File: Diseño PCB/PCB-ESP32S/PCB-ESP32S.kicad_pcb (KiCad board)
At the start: 2 copper layers, 29 parts, among them J1 Conn_01x04, J7 Screw_Terminal_01x03, J8 Screw_Terminal_01x02, Q3 TIP42C, SW1 SW_DIP_x01, SW2 SW_DIP_x01, U1 ESP-32S, U5 LM7805_TO220, U6 LM1117-3.3, u2 Conn_01x04_Male, u7 Conn_01x04_Male

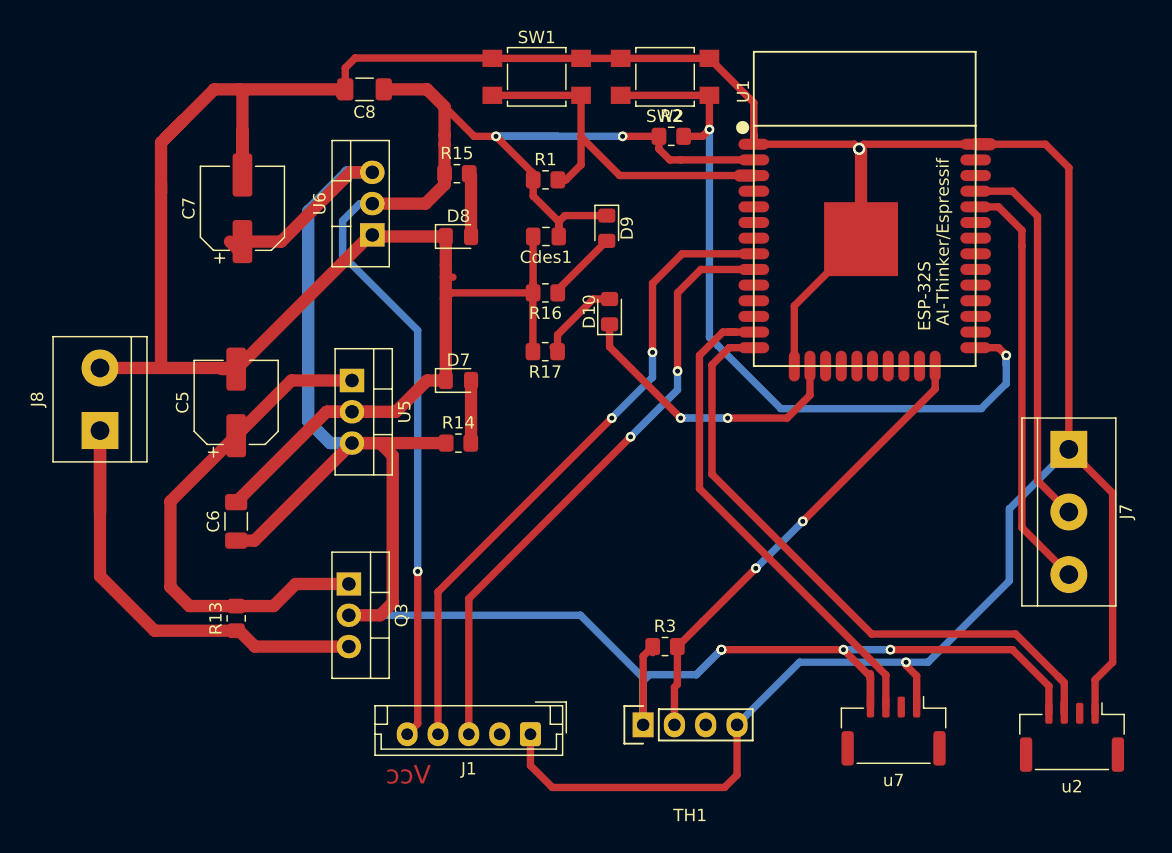
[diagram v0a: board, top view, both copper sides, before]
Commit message: pcv v2
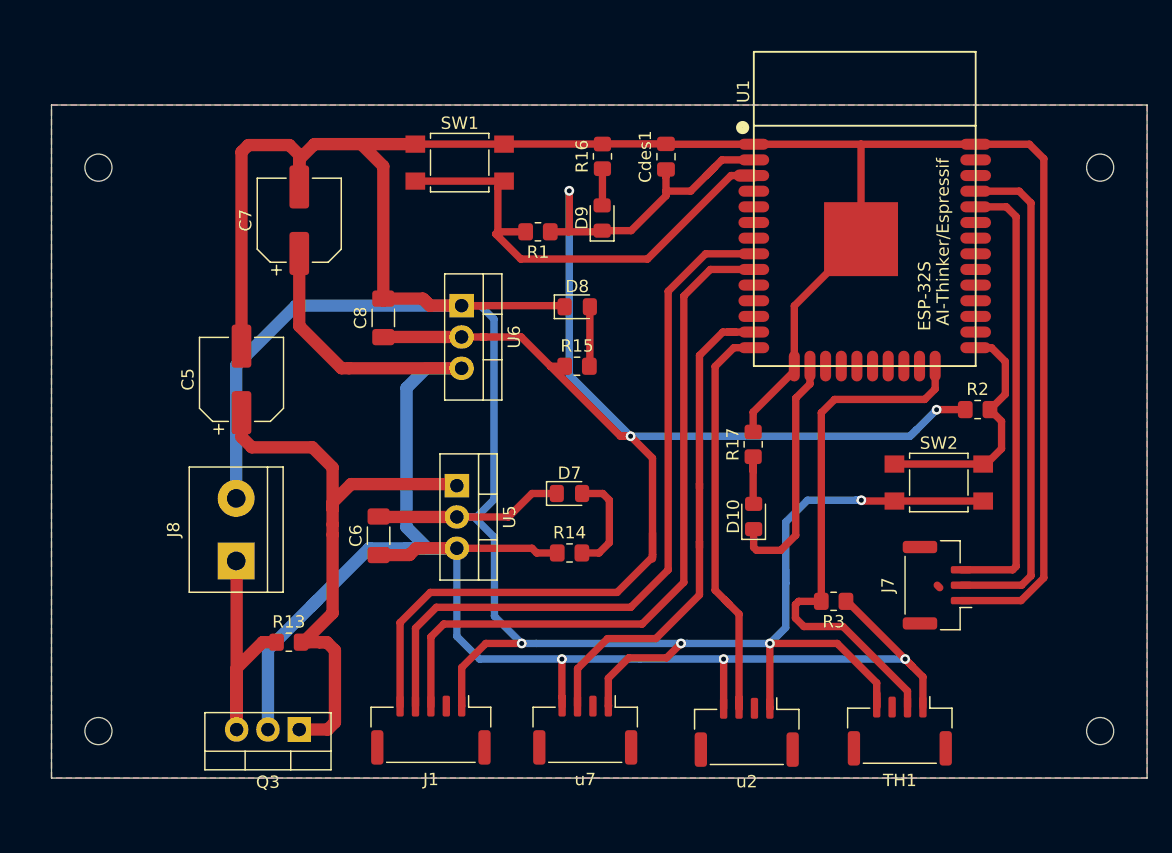
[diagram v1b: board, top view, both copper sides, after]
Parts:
- added ?: MountingHole_2.2mm_M2, MountingHole:MountingHole_2.2mm_M2, F.Cu at (243.8, 80.0)
- added ?: MountingHole_2.2mm_M2, MountingHole:MountingHole_2.2mm_M2, F.Cu at (243.8, 125.7)
- added ?: MountingHole_2.2mm_M2, MountingHole:MountingHole_2.2mm_M2, F.Cu at (162.6, 125.7)
- added ?: MountingHole_2.2mm_M2, MountingHole:MountingHole_2.2mm_M2, F.Cu at (162.6, 80.0)
- J1: footprint Connector_JST:JST_EH_B5B-EH-A_1x05_P2.50mm_Vertical -> Connector_JST:JST_GH_BM05B-GHS-TBT_1x05-1MP_P1.25mm_Vertical
- J7: footprint TerminalBlock:TerminalBlock_bornier-3_P5.08mm -> Connector_JST:JST_GH_BM03B-GHS-TBT_1x03-1MP_P1.25mm_Vertical
- TH1: footprint Sensors:DHT22_Temperature_Humidity -> Connector_JST:JST_GH_BM04B-GHS-TBT_1x04-1MP_P1.25mm_Vertical
- moved SW2 39.7 mm to (230.7, 105.6), turned to 0 degrees
- moved R2 33.3 mm to (233.9, 99.6)
- moved u2 26.4 mm to (215.2, 125.8)
- moved u7 25.0 mm to (202.1, 125.7)
- moved D10 20.3 mm to (215.7, 108.3)
- moved C8 18.6 mm to (185.7, 92.2), turned to 90 degrees
- moved R17 18.5 mm to (215.7, 102.5), turned to 90 degrees
- moved R15 18.4 mm to (201.4, 96.1)
- moved TH1 17.0 mm to (227.6, 125.7), turned to 180 degrees
- moved J7 15.3 mm to (230.6, 113.9), turned to 90 degrees
- moved J8 15.3 mm to (173.7, 111.9)
- moved R3 14.2 mm to (222.2, 115.2), turned to 180 degrees
- moved D7 12.9 mm to (200.8, 106.5)
- moved R14 12.7 mm to (200.8, 111.3)
- moved Q3 12.5 mm to (178.9, 125.6), turned to 180 degrees
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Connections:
- J1 pad 2: /BH1750/ADDR -> (no net)
- TH1 pad 3: Net-(TH1-Pad3) -> (no net)
- U1 pad 10: Net-(U1-Pad10) -> (no net)
- U1 pad 11: Net-(U1-Pad11) -> (no net)
- U1 pad 12: Net-(U1-Pad12) -> (no net)
- U1 pad 17: Net-(U1-Pad17) -> (no net)
- U1 pad 18: Net-(U1-Pad18) -> (no net)
- U1 pad 19: Net-(U1-Pad19) -> (no net)
- U1 pad 20: Net-(U1-Pad20) -> (no net)
- U1 pad 21: Net-(U1-Pad21) -> (no net)
- U1 pad 22: Net-(U1-Pad22) -> (no net)
- U1 pad 23: Net-(U1-Pad23) -> (no net)
- U1 pad 26: Net-(U1-Pad26) -> (no net)
- U1 pad 27: Net-(U1-Pad27) -> (no net)
- U1 pad 28: Net-(U1-Pad28) -> (no net)
- U1 pad 29: Net-(U1-Pad29) -> (no net)
- U1 pad 30: Net-(U1-Pad30) -> (no net)
- U1 pad 31: Net-(U1-Pad31) -> (no net)
- U1 pad 32: Net-(U1-Pad32) -> (no net)
- U1 pad 33: Net-(U1-Pad33) -> (no net)
- U1 pad 36: Net-(U1-Pad36) -> (no net)
- U1 pad 37: Net-(U1-Pad37) -> (no net)
- U1 pad 4: Net-(U1-Pad4) -> (no net)
- U1 pad 5: Net-(U1-Pad5) -> (no net)
- U1 pad 6: Net-(U1-Pad6) -> (no net)
- U1 pad 7: Net-(U1-Pad7) -> (no net)
- u2 pad 2: Net-(u2-Pad2) -> (no net)
- u7 pad 2: Net-(u7-Pad2) -> (no net)
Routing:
- net Net-(R2-Pad2): track 62.3 -> 20.1 mm, vias 2 -> 0
- net +3V3: track 116.8 -> 144.1 mm
- net IO12: track 52.3 -> 33.6 mm
- net +5V: track 168.3 -> 150.2 mm, vias 4 -> 3
- net /Sheet61A8C81E/12v: track 41.1 -> 23.0 mm
- net GND: track 344.1 -> 355.9 mm, vias 2 -> 4
- net Net-(J7-Pad2): track 30.9 -> 41.1 mm
- net Net-(C5-Pad1): track 41.6 -> 50.3 mm
- net Net-(R1-Pad2): track 31.7 -> 39.8 mm
- net IO33: track 49.8 -> 57.8 mm, vias 2 -> 0
- net IO32: track 53.0 -> 59.6 mm, vias 2 -> 0
- net IO2: track 37.9 -> 43.4 mm, vias 2 -> 0
- net Net-(D10-Pad1): track 23.6 -> 19.7 mm, vias 2 -> 0
- net Net-(D7-Pad2): track 5.09 -> 8.52 mm
- net Net-(D9-Pad2): track 6.11 -> 2.99 mm
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- added copper zone on B.Cu, net GND
- added copper zone on F.Cu, net GND
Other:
- board outline added: 88.9 x 54.6 mm
- rule trace_min: 0.2 -> 0
- rule via_min_size: 0.4 -> 0.8
- board text removed: "Vcc"
